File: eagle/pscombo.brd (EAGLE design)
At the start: 152.9 x 196.8 mm, 32 parts, among them J1 PIN2F061.100, J2 PIN2F061.100

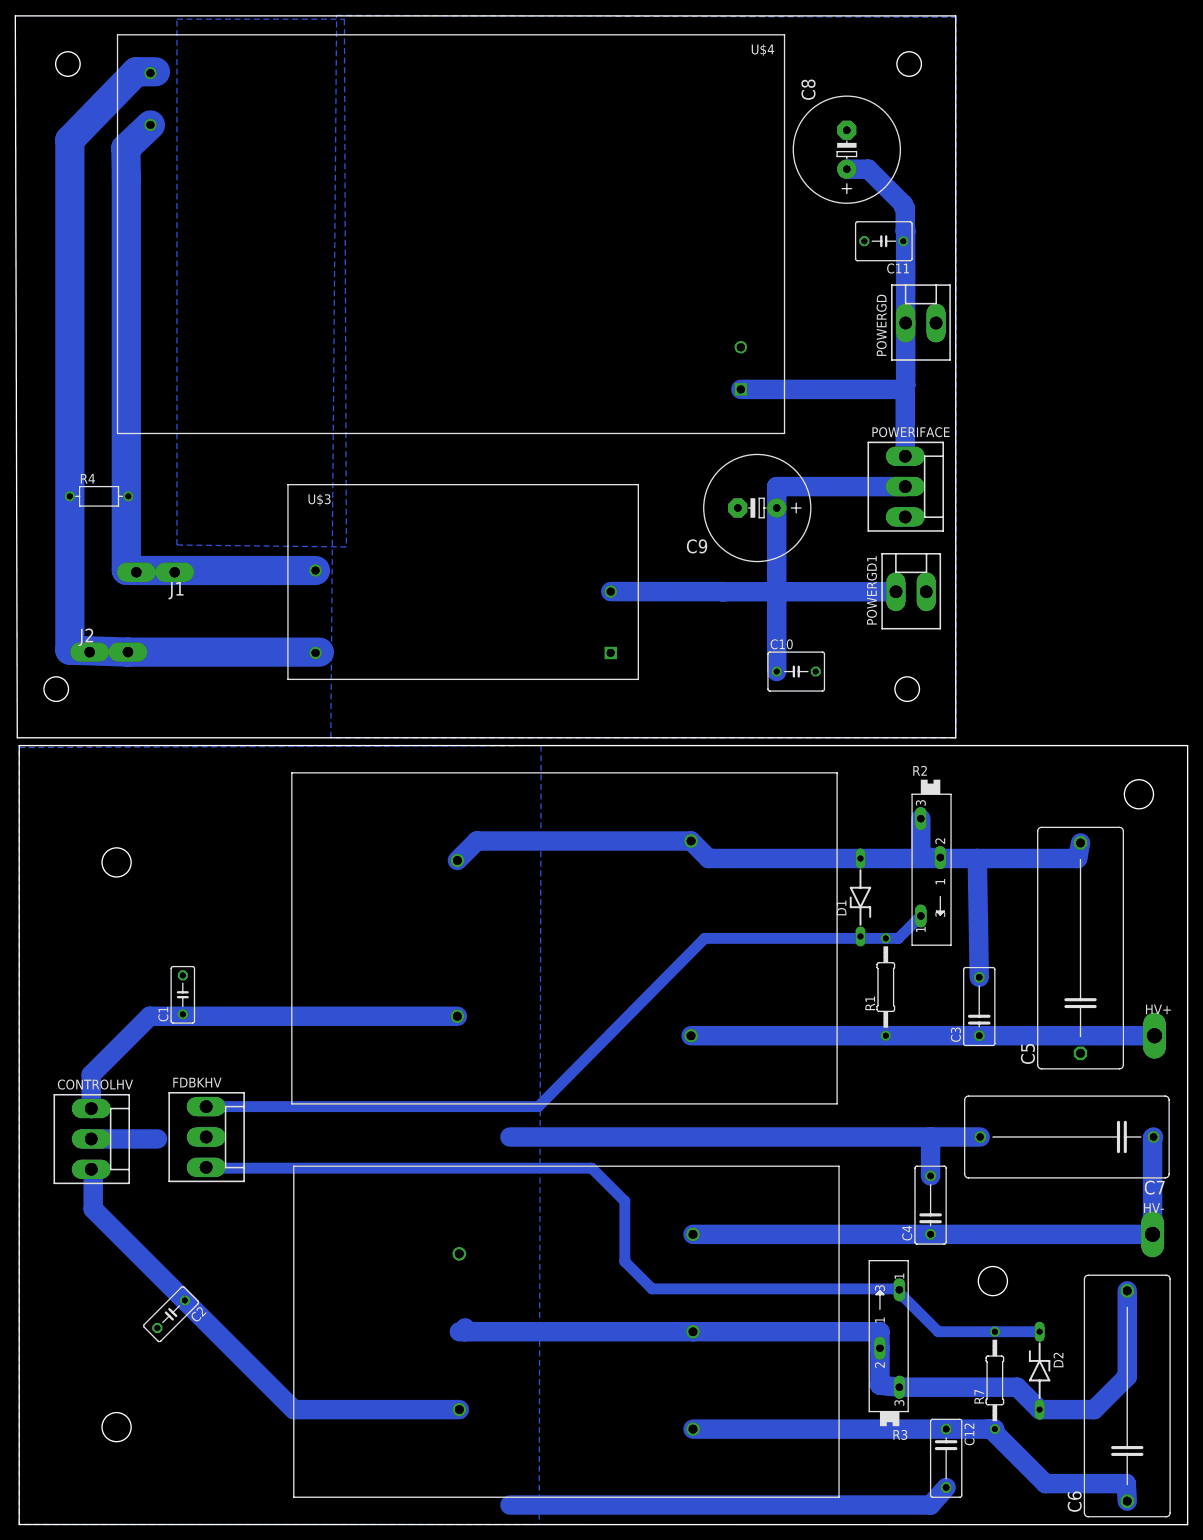
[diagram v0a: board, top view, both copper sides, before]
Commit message: IXYS board solution, gatedriver components
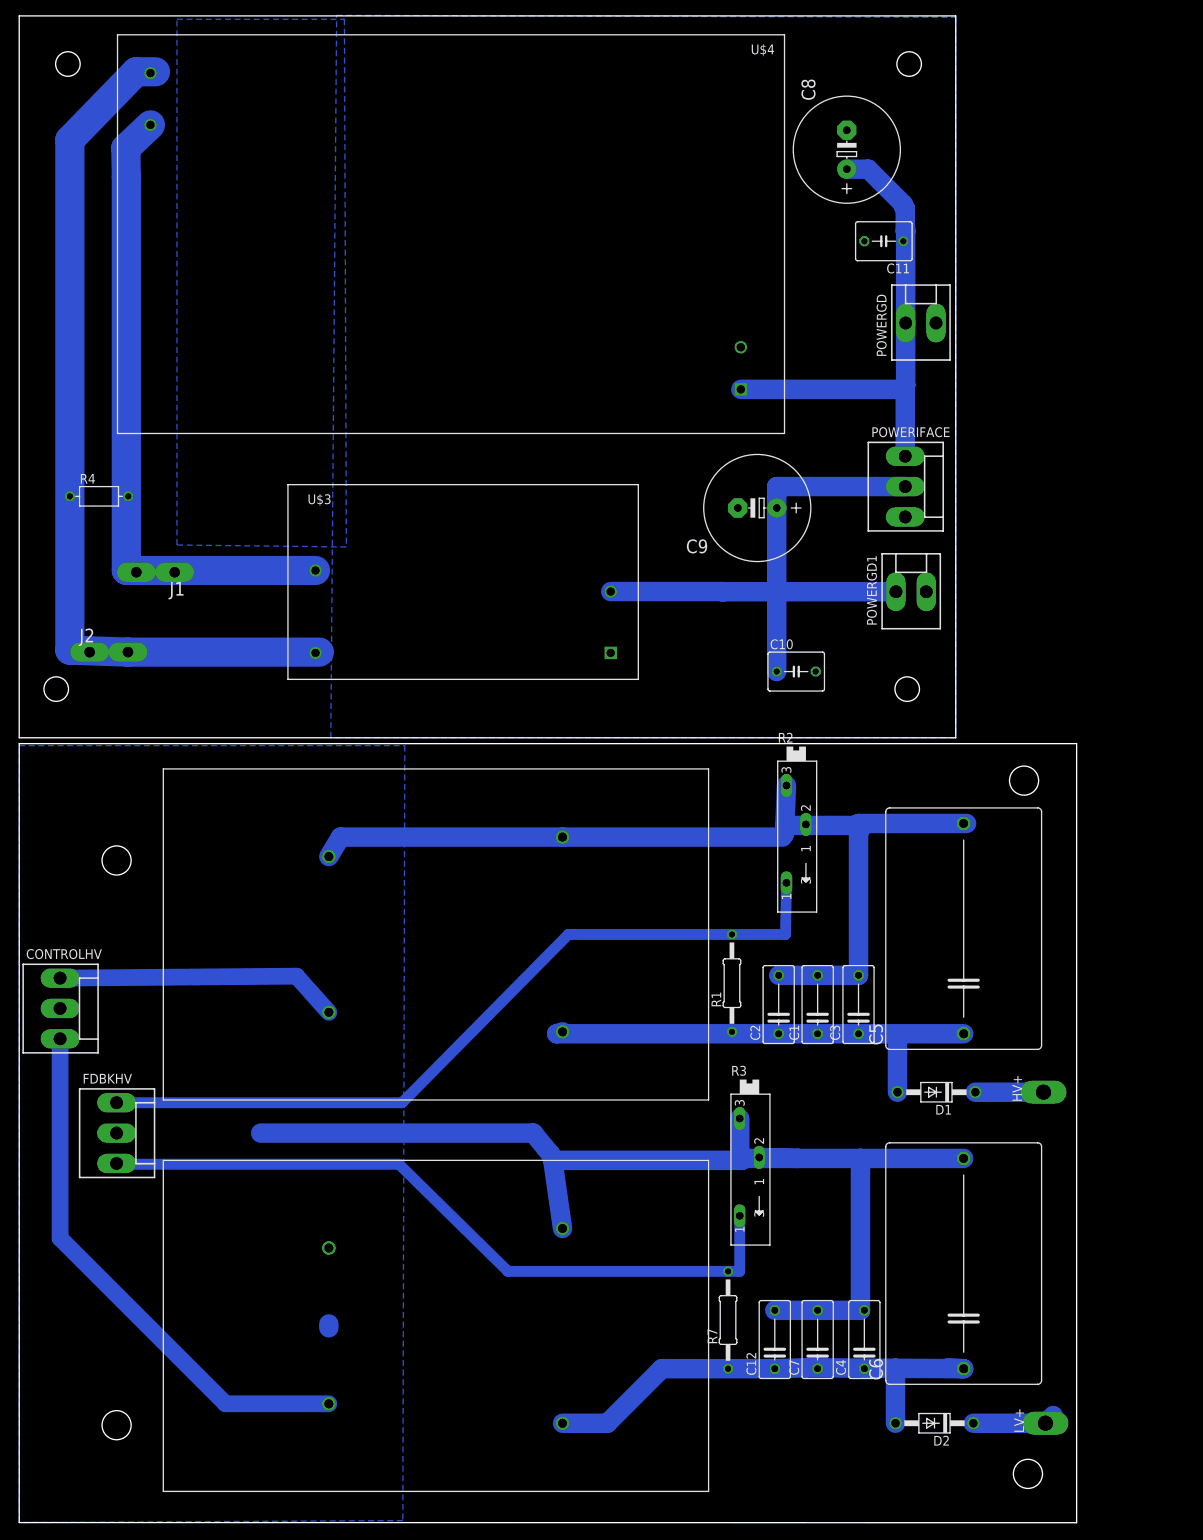
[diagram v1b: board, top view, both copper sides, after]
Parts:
- removed HV-: TPPAD1-20Y, testpad:P1-20Y
- added LV+: TPPAD1-20Y, testpad:P1-20Y
- C1: value (none) -> 1n; device rcl:C050-030X075 -> rcl:C075-042X103
- C2: value (none) -> 10p; device rcl:C050-030X075 -> rcl:C075-042X103
- C4: value .01u -> 1n
- C5, C6: device rcl:C275-113X316 -> rcl:C275-205X316
- C7: value 1u -> 10p; device rcl:C225-108X268 -> rcl:C075-042X103
- D1, D2: value 1n4733 -> 1N4004; device diode:ZDIO-10 -> diode:DO41-10
- U$2: value EMCO-F20CT -> EMCO-F104PIN; device dc-dc-converter:EMCO-F*CT -> dc-dc-converter:EMCO-F
- moved C2 88.9 mm to (99.1, 67.8), turned to 90 degrees
- moved C1 82.8 mm to (104.1, 67.8)
- moved C7 41.9 mm to (104.1, 24.1), turned to 90 degrees
- moved R7 35.7 mm to (92.5, 26.7)
- moved R3 27.9 mm to (95.2, 46.0), turned to 270 degrees
- moved C6 27.5 mm to (123.2, 34.0)
- moved D1 27.3 mm to (119.6, 56.4), turned to 180 degrees
- moved C12 27.2 mm to (98.6, 24.1), turned to 90 degrees
- moved R1 20.1 mm to (93.0, 70.6)
- moved C4 19.5 mm to (110.2, 24.1)
- moved R2 18.1 mm to (101.3, 89.4)
- moved CONTROLHV 17.5 mm to (5.33, 67.3)
- moved U$2 17.0 mm to (40.4, 15.7)
- moved U$1 16.8 mm to (40.4, 66.8)
- moved HV+ 16.2 mm to (133.6, 56.4), turned to 90 degrees
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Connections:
- new net N$7: D2.C, LV+.TP
- net GND: now also U$2.P$4; no longer D1.A, D2.A, U$2.P$5
- net N$1: now also C1.1, C2.1, D1.A; no longer HV+.TP
- net N$2: now also C4.1, C7.1, D2.A
- net N$3: no longer D1.C
- net N$4: no longer C1.1
- net N$5: no longer C2.1
- net N$6: now also D1.C, HV+.TP; no longer C4.1, C7.1, HV-.TP, U$2.P$4
- net N$8: no longer D2.C
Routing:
- net GND: track 349.9 -> 267.2 mm
- net N$6: track 72.7 -> 10.2 mm
- net N$8: track 122.2 -> 95.1 mm
- net N$4: track 55.3 -> 37.2 mm
- net N$7: track 0.00 -> 10.8 mm
- net N$5: track 63.9 -> 70.0 mm
- net N$2: track 62.3 -> 64.5 mm
- net N$1: track 60.5 -> 61.0 mm
- added copper zone on layer 16, net N$11
- removed copper zone on layer 16, net N$10 (its old number)
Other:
- board size 152.9 x 196.8 mm -> 137.9 x 196.5 mm
